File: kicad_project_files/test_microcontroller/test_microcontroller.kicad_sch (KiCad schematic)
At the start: 39 parts, among them J1 USB_C_Receptacle_USB2.0, SW1 SW_Push, SW2 SW_Push, SW3 SW_Push, SW4 SW_Push, SW5 SW_Push, SW6 SW_Push, SW7 SW_Push, SW8 SW_Push, SW9 SW_Push, U1 ATmega32U4-A, Y1 16mhz

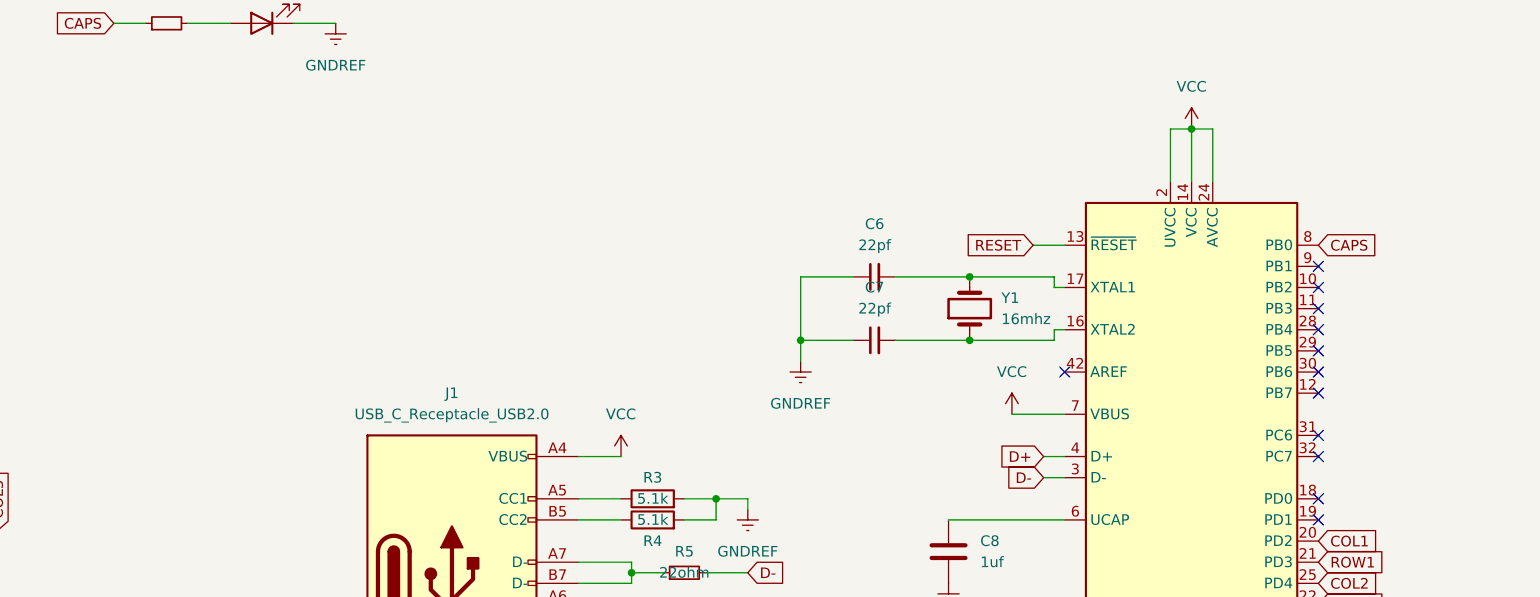
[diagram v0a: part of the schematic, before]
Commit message: add ICSP
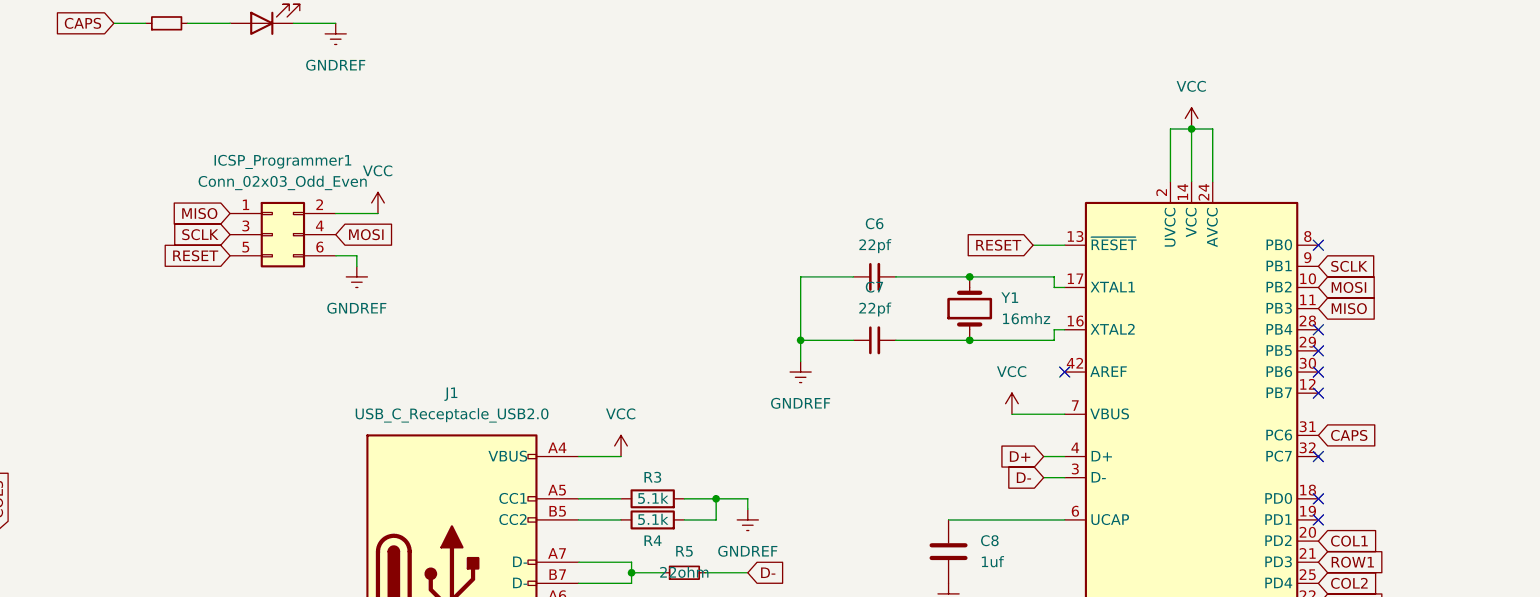
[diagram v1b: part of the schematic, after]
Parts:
- added ICSP_Programmer1: Conn_02x03_Odd_Even, Connector_PinHeader_2.00mm:PinHeader_2x03_P2.00mm_Vertical, symbol Connector_Generic:Conn_02x03_Odd_Even
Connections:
- net CAPS: now also U1.31 (PC6); no longer U1.8 (PB0)
- net GNDREF: now also ICSP_Programmer1.2 (Pin_2), ICSP_Programmer1.6 (Pin_6)
- net RESET: now also ICSP_Programmer1.5 (Pin_5)
- net MOSI: now reaches U1.10 (PB2)
- net MOSI: now also ICSP_Programmer1.4 (Pin_4)
- net MISO: now reaches U1.11 (PB3)
- net MISO: now also ICSP_Programmer1.1 (Pin_1)
- net SCLK: now reaches U1.9 (PB1)
- net SCLK: now also ICSP_Programmer1.3 (Pin_3)
- no-connect marks 21 -> 18
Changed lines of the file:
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@@
   (no_connect (at 246.38 82.55))
   (no_connect (at 246.38 80.01))
-  (no_connect (at 246.38 72.39))
   (no_connect (at 246.38 74.93))
-  (no_connect (at 246.38 52.07))
-  (no_connect (at 246.38 54.61))
-  (no_connect (at 246.38 57.15))
   (no_connect (at 246.38 59.69))
   (no_connect (at 246.38 120.65))
@@
   (no_connect (at 246.38 67.31))
   (no_connect (at 246.38 105.41))
+  (no_connect (at 246.38 49.53))
+  (wire (pts (xy 130.81 50.8) (xy 130.81 52.07))
+    (stroke (width 0) (type default) (color 0 0 0 0))
+  )
   (wire (pts (xy 24.13 19.05) (xy 24.13 21.59))
     (stroke (width 0) (type default) (color 0 0 0 0))
@@
     (stroke (width 0) (type default) (color 0 0 0 0))
   )
+  (wire (pts (xy 128.27 50.8) (xy 130.81 50.8))
+    (stroke (width 0) (type default) (color 0 0 0 0))
+  )
   (wire (pts (xy 233.68 35.56) (xy 231.14 35.56))
     (stroke (width 0) (type default) (color 0 0 0 0))
@@
   )
   (wire (pts (xy 163.83 90.17) (xy 163.83 88.9))
+    (stroke (width 0) (type default) (color 0 0 0 0))
+  )
+  (wire (pts (xy 128.27 45.72) (xy 133.35 45.72))
     (stroke (width 0) (type default) (color 0 0 0 0))
   )
@@
     )
   )
-  (global_label "CAPS" (shape input) (at 246.38 49.53 0) (fields_autoplaced)
+  (global_label "SCLK" (shape input) (at 115.57 48.26 180) (fields_autoplaced)
+    (effects (font (size 1.27 1.27)) (justify right))
+    (property "Intersheet References" "${INTERSHEET_REFS}" (id 0) (at 108.3793 48.3394 0)
+      (effects (font (size 1.27 1.27)) (justify right) hide)
+    )
+  )
+  (global_label "CAPS" (shape input) (at 246.38 72.39 0) (fields_autoplaced)
     (effects (font (size 1.27 1.27)) (justify left))
-    (property "Intersheet References" "${INTERSHEET_REFS}" (id 0) (at 253.6312 49.6094 0)
+    (property "Intersheet References" "${INTERSHEET_REFS}" (id 0) (at 253.6312 72.4694 0)
       (effects (font (size 1.27 1.27)) (justify left) hide)
     )
@@
     )
   )
+  (global_label "RESET" (shape input) (at 115.57 50.8 180) (fields_autoplaced)
+    (effects (font (size 1.27 1.27)) (justify right))
+    (property "Intersheet References" "${INTERSHEET_REFS}" (id 0) (at 107.4117 50.7206 0)
+      (effects (font (size 1.27 1.27)) (justify right) hide)
+    )
+  )
   (global_label "D-" (shape input) (at 213.36 77.47 180) (fields_autoplaced)
     (effects (font (size 1.27 1.27)) (justify right))
@@
     )
   )
+  (global_label "MOSI" (shape input) (at 128.27 48.26 0) (fields_autoplaced)
+    (effects (font (size 1.27 1.27)) (justify left))
+    (property "Intersheet References" "${INTERSHEET_REFS}" (id 0) (at 135.2793 48.1806 0)
+      (effects (font (size 1.27 1.27)) (justify left) hide)
+    )
+  )
   (global_label "CAPS" (shape input) (at 101.6 22.86 180) (fields_autoplaced)
     (effects (font (size 1.27 1.27)) (justify right))
@@
     )
   )
+  (global_label "SCLK" (shape input) (at 246.38 52.07 0) (fields_autoplaced)
+    (effects (font (size 1.27 1.27)) (justify left))
+    (property "Intersheet References" "${INTERSHEET_REFS}" (id 0) (at 253.5707 51.9906 0)
+      (effects (font (size 1.27 1.27)) (justify left) hide)
+    )
+  )
   (global_label "ROW1" (shape input) (at 33.02 106.68 180) (fields_autoplaced)
     (effects (font (size 1.27 1.27)) (justify right))
@@
     (effects (font (size 1.27 1.27)) (justify left))
     (property "Intersheet References" "${INTERSHEET_REFS}" (id 0) (at 254.0545 97.8694 0)
+      (effects (font (size 1.27 1.27)) (justify left) hide)
+    )
+  )
+  (global_label "MISO" (shape input) (at 115.57 45.72 180) (fields_autoplaced)
+    (effects (font (size 1.27 1.27)) (justify right))
+    (property "Intersheet References" "${INTERSHEET_REFS}" (id 0) (at 108.5607 45.7994 0)
+      (effects (font (size 1.27 1.27)) (justify right) hide)
+    )
+  )
+  (global_label "MOSI" (shape input) (at 246.38 54.61 0) (fields_autoplaced)
+    (effects (font (size 1.27 1.27)) (justify left))
+    (property "Intersheet References" "${INTERSHEET_REFS}" (id 0) (at 253.3893 54.5306 0)
+      (effects (font (size 1.27 1.27)) (justify left) hide)
+    )
+  )
+  (global_label "MISO" (shape input) (at 246.38 57.15 0) (fields_autoplaced)
+    (effects (font (size 1.27 1.27)) (justify left))
+    (property "Intersheet References" "${INTERSHEET_REFS}" (id 0) (at 253.3893 57.0706 0)
       (effects (font (size 1.27 1.27)) (justify left) hide)
     )
@@
     (pin "2")
   )
+  (symbol (lib_id "Connector_Generic:Conn_02x03_Odd_Even") (at 120.65 48.26 0) (unit 1)
+    (in_bom yes) (on_board yes) (fields_autoplaced)
+    (property "Reference" "ICSP_Programmer1" (id 0) (at 121.92 39.37 0))
+    (property "Value" "Conn_02x03_Odd_Even" (id 1) (at 121.92 41.91 0))
+    (property "Footprint" "Connector_PinHeader_2.00mm:PinHeader_2x03_P2.00mm_Vertical" (id 2) (at 120.65 48.26 0)
+      (effects (font (size 1.27 1.27)) hide)
+    )
+    (property "Datasheet" "~" (id 3) (at 120.65 48.26 0)
+      (effects (font (size 1.27 1.27)) hide)
+    )
+    (pin "1")
+    (pin "2")
+    (pin "3")
+    (pin "4")
+    (pin "5")
+    (pin "6")
+  )
   (symbol (lib_id "power:GNDREF") (at 16.51 57.15 0) (unit 1)
     (in_bom yes) (on_board yes) (fields_autoplaced)
@@
     (pin "1")
     (pin "2")
+  )
+  (symbol (lib_id "power:VCC") (at 133.35 45.72 0) (unit 1)
+    (in_bom yes) (on_board yes) (fields_autoplaced)
+    (property "Reference" "#PWR017" (id 0) (at 133.35 49.53 0)
+      (effects (font (size 1.27 1.27)) hide)
+    )
+    (property "Value" "VCC" (id 1) (at 133.35 40.64 0))
+    (property "Footprint" "" (id 2) (at 133.35 45.72 0)
+      (effects (font (size 1.27 1.27)) hide)
+    )
+    (property "Datasheet" "" (id 3) (at 133.35 45.72 0)
+      (effects (font (size 1.27 1.27)) hide)
+    )
+    (pin "1")
   )
   (symbol (lib_id "Diode:1N4148") (at 77.47 124.46 90) (unit 1)
@@
     (pin "1")
   )
+  (symbol (lib_id "power:GNDREF") (at 130.81 52.07 0) (unit 1)
+    (in_bom yes) (on_board yes) (fields_autoplaced)
+    (property "Reference" "#PWR016" (id 0) (at 130.81 58.42 0)
+      (effects (font (size 1.27 1.27)) hide)
+    )
+    (property "Value" "GNDREF" (id 1) (at 130.81 57.15 0))
+    (property "Footprint" "" (id 2) (at 130.81 52.07 0)
+      (effects (font (size 1.27 1.27)) hide)
+    )
+    (property "Datasheet" "" (id 3) (at 130.81 52.07 0)
+      (effects (font (size 1.27 1.27)) hide)
+    )
+    (pin "1")
+  )
   (symbol (lib_id "power:VCC") (at 231.14 35.56 0) (unit 1)
     (in_bom yes) (on_board yes) (fields_autoplaced)
@@
   (symbol (lib_id "power:GNDREF") (at 64.77 21.59 0) (unit 1)
     (in_bom yes) (on_board yes) (fields_autoplaced)
-    (property "Reference" "#PWR?" (id 0) (at 64.77 27.94 0)
+    (property "Reference" "#PWR015" (id 0) (at 64.77 27.94 0)
       (effects (font (size 1.27 1.27)) hide)
     )
@@
       (reference "#PWR014") (unit 1) (value "GNDREF") (footprint "")
     )
+    (path "/f70e8927-2299-449c-b52c-553c1bc34b5d"
+      (reference "#PWR015") (unit 1) (value "GNDREF") (footprint "")
+    )
+    (path "/6f9440f8-a9f0-42af-bfc6-f816927170e2"
+      (reference "#PWR016") (unit 1) (value "GNDREF") (footprint "")
+    )
+    (path "/25d8ce34-f34b-4496-8900-e9d2598324a2"
+      (reference "#PWR017") (unit 1) (value "VCC") (footprint "")
+    )
     (path "/a717bee7-1902-40ae-b673-fad1ccbf129c"
       (reference "#PWR0101") (unit 1) (value "GNDREF") (footprint "")
@@
       (reference "#PWR0102") (unit 1) (value "VCC") (footprint "")
     )
-    (path "/f70e8927-2299-449c-b52c-553c1bc34b5d"
-      (reference "#PWR?") (unit 1) (value "GNDREF") (footprint "")
-    )
     (path "/4d48e41d-3878-4a27-ab4f-51a7ebfea6fe"
       (reference "C1") (unit 1) (value "0.1uf") (footprint "Capacitor_THT:C_Disc_D3.0mm_W1.6mm_P2.50mm")
@@
       (reference "D_CAPS1") (unit 1) (value "LED") (footprint "LED_THT:LED_D3.0mm")
     )
+    (path "/1bc5dd36-6c22-4532-936b-9ec262629ce9"
+      (reference "ICSP_Programmer1") (unit 1) (value "Conn_02x03_Odd_Even") (footprint "Connector_PinHeader_2.00mm:PinHeader_2x03_P2.00mm_Vertical")
+    )
     (path "/29e44f23-b958-4c15-8e4c-23c54ef10f8f"
